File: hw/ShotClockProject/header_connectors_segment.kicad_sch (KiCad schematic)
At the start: 4 parts, among them J10 DW254W-22-20-85, J7 DW254W-22-20-85, J8 DW254W-22-20-85, J9 DW254W-22-20-85

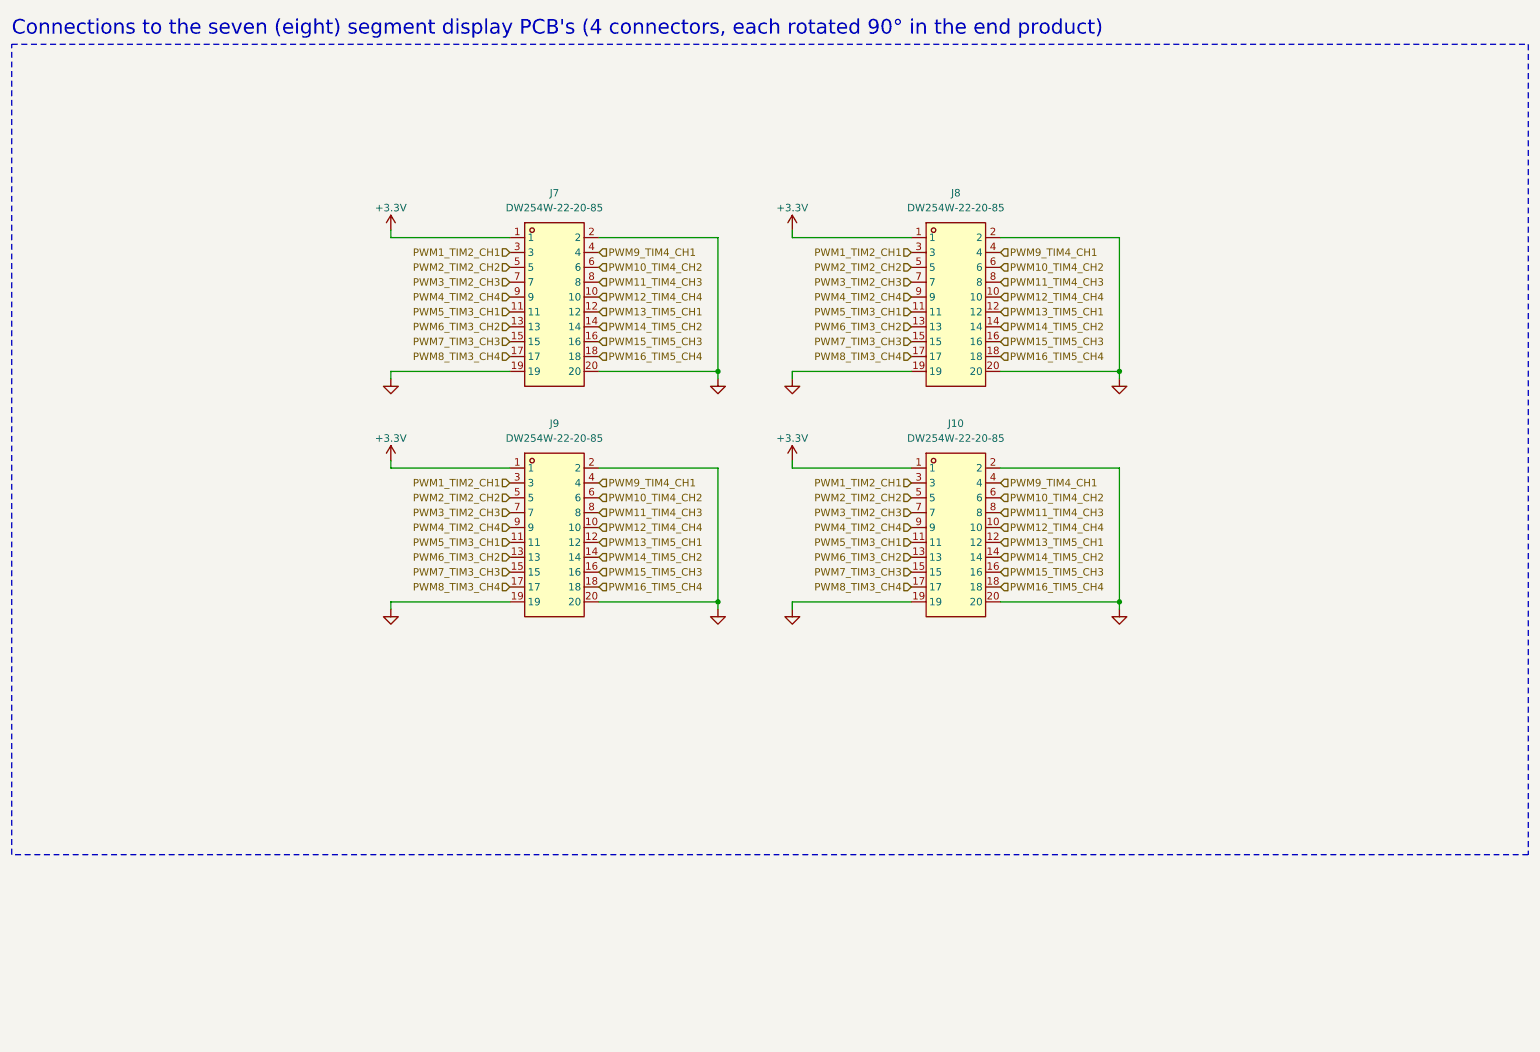
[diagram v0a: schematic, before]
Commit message: First feedback round from Luc on schematic
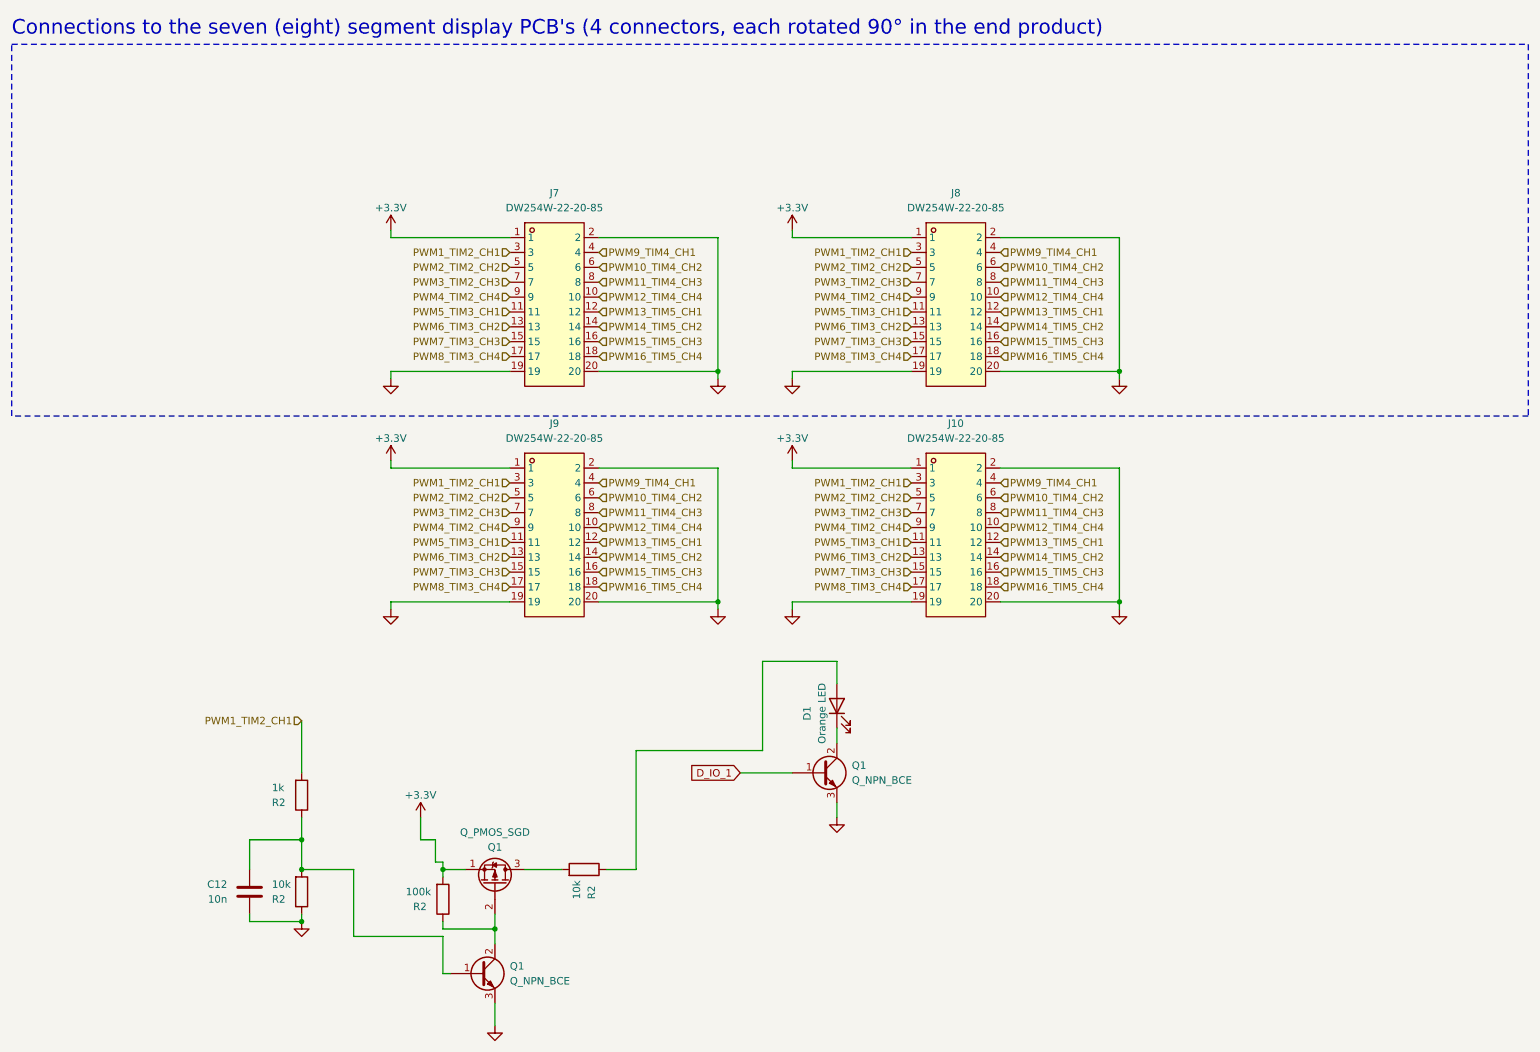
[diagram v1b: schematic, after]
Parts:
- added C12: 10n, Capacitor_SMD:C_0603_1608Metric, symbol Device:C
- added D1: Orange LED, LED_SMD:LED_0603_1608Metric, symbol Device:LED
- added Q1 (x2): Q_NPN_BCE, Package_TO_SOT_SMD:SOT-23, symbol Device:Q_NPN_BCE
- added Q1: Q_PMOS_SGD, symbol Device:Q_PMOS_SGD
- added R2: 1k, Resistor_SMD:R_0402_1005Metric, symbol Device:R
- added R2 (x2): 10k, Resistor_SMD:R_0402_1005Metric, symbol Device:R
- added R2: 100k, Resistor_SMD:R_0402_1005Metric, symbol Device:R
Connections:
- net +3.3V: now also Q1.1 (S), R2.2
- net GND: now also C12.2, Q1.3 (E), Q1.3 (E), R2.1
- net PWM1_TIM2_CH1: now also R2.2
- new net: C12.1, Q1.1 (B), R2.1, R2.2
- new net: Q1.2 (C), Q1.2 (G), R2.1
- new net: D1.1 (K), Q1.2 (C)
- new net: D1.2 (A), R2.1
- new net: Q1.3 (D), R2.2
- new net D_IO_1: Q1.1 (B)
